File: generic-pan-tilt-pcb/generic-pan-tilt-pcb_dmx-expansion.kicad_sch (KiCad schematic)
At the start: 3 parts, among them J11 Conn_01x08, J12 Conn_01x08, J13 Conn_01x05

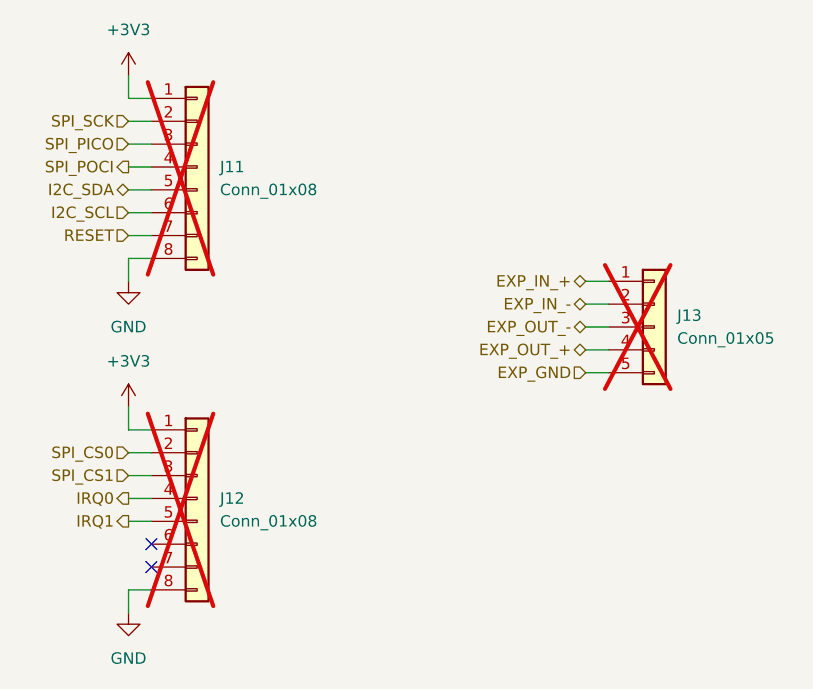
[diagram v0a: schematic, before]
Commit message: begin new routing
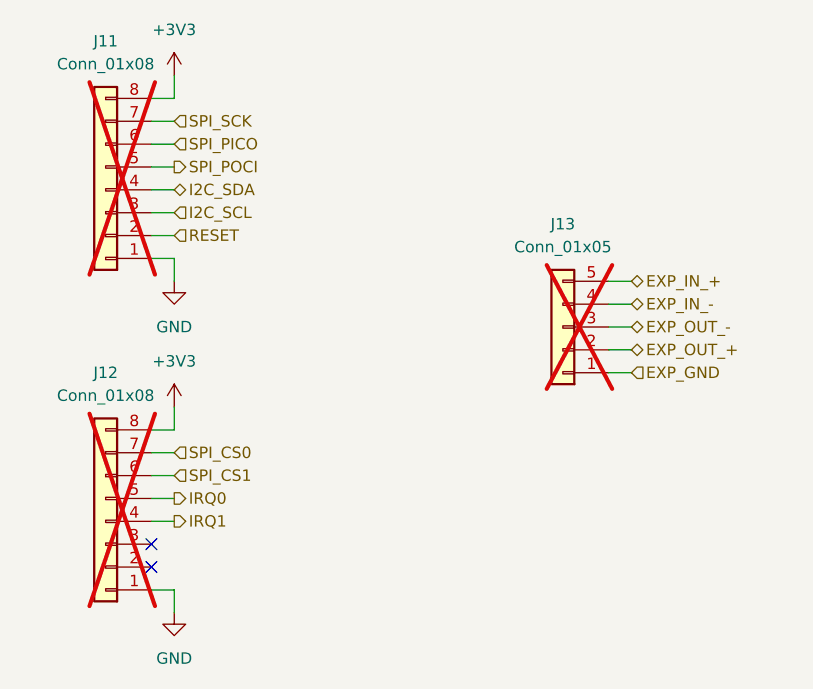
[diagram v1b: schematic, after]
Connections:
- net +3V3: now also J11.8 (Pin_8), J12.8 (Pin_8); no longer J11.1 (Pin_1), J12.1 (Pin_1)
- net EXP_GND: now also J13.1 (Pin_1); no longer J13.5 (Pin_5)
- net EXP_IN_+: now also J13.5 (Pin_5); no longer J13.1 (Pin_1)
- net EXP_IN_-: now also J13.4 (Pin_4); no longer J13.2 (Pin_2)
- net EXP_OUT_+: now also J13.2 (Pin_2); no longer J13.4 (Pin_4)
- net GND: now also J11.1 (Pin_1), J12.1 (Pin_1); no longer J11.8 (Pin_8), J12.8 (Pin_8)
- net I2C_SCL: now also J11.3 (Pin_3); no longer J11.6 (Pin_6)
- net I2C_SDA: now also J11.4 (Pin_4); no longer J11.5 (Pin_5)
- net IRQ0: now also J12.5 (Pin_5); no longer J12.4 (Pin_4)
- net IRQ1: now also J12.4 (Pin_4); no longer J12.5 (Pin_5)
- net RESET: now also J11.2 (Pin_2); no longer J11.7 (Pin_7)
- net SPI_CS0: now also J12.7 (Pin_7); no longer J12.2 (Pin_2)
- net SPI_CS1: now also J12.6 (Pin_6); no longer J12.3 (Pin_3)
- net SPI_PICO: now also J11.6 (Pin_6); no longer J11.3 (Pin_3)
- net SPI_POCI: now also J11.5 (Pin_5); no longer J11.4 (Pin_4)
- net SPI_SCK: now also J11.7 (Pin_7); no longer J11.2 (Pin_2)
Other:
- moved on the sheet: J11, J12, J13
